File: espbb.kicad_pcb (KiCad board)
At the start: 2 copper layers, 20 x 20 mm, 10 parts, among them P1 CONN_8, P2 CONN_8, SW1 SWITCH_INV, U1 ESP-12/07v2/08v2, U2 LM6206

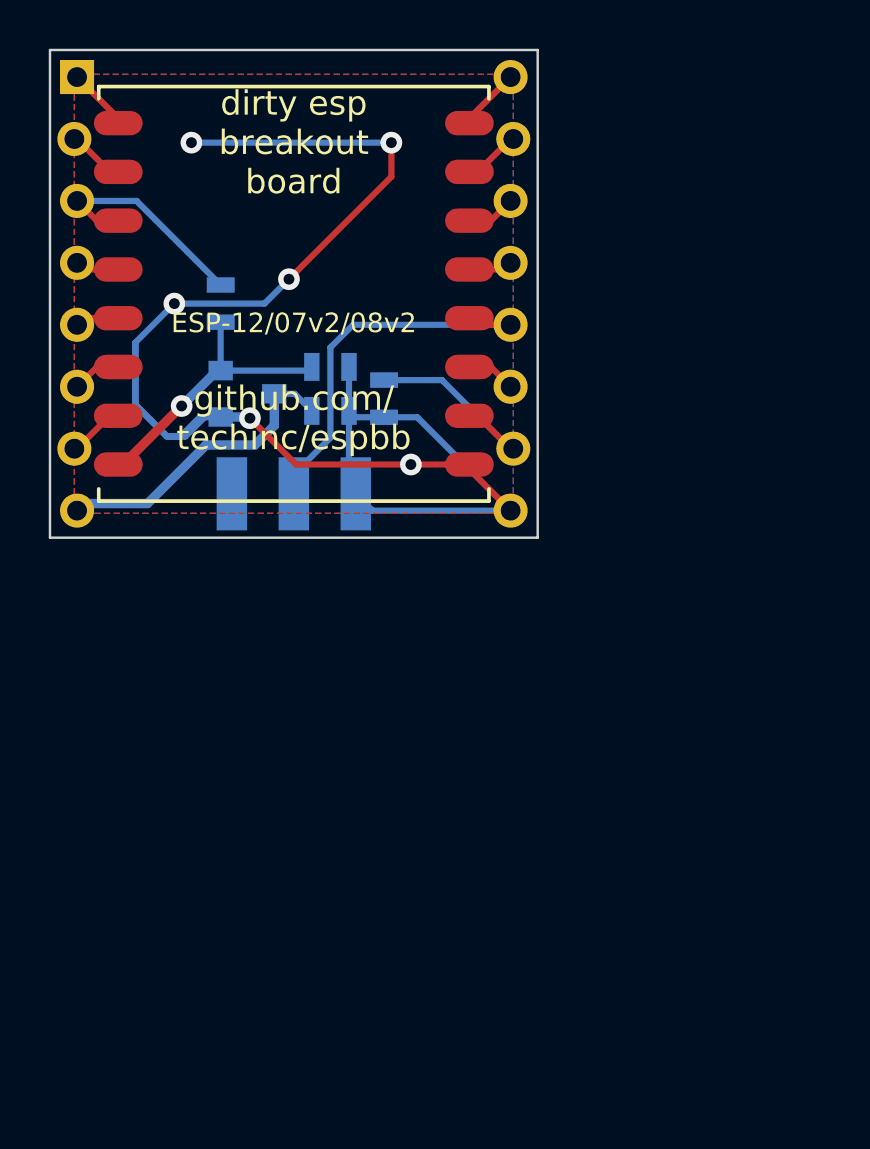
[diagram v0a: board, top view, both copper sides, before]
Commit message: esp-12e version
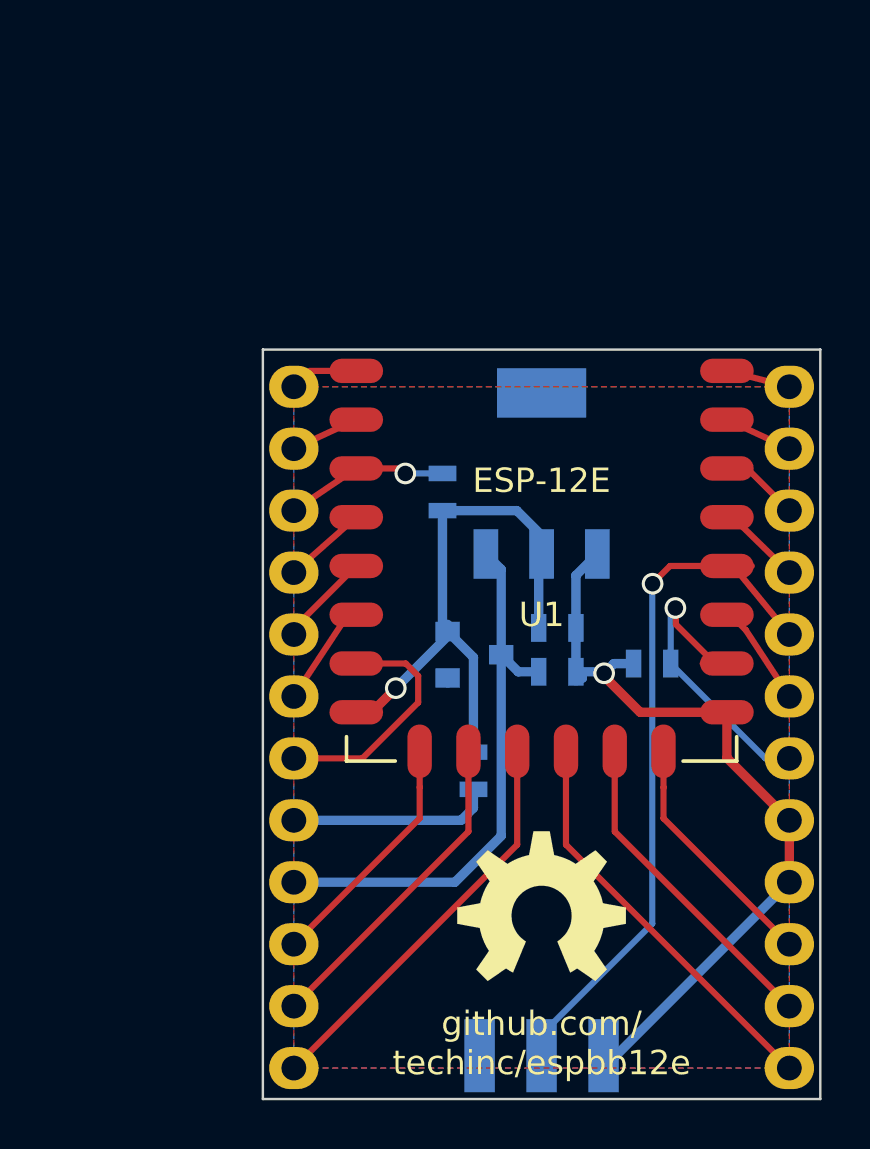
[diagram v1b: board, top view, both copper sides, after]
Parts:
- added R3: 0Ohm, r0603:SM0603, B.Cu at (7.37, 19.6)
- added U3: AMS1117-3.3, sot223:SOT223, B.Cu at (10.2, 7.37)
- ?: moved to F.Cu
- P1, P2: value CONN_8 -> CONN_01X12; footprint SIL-8 -> Pin_Headers:Pin_Header_Straight_1x12
- U1: value ESP-12/07v2/08v2 -> ESP-12E; footprint ESP-08v2 -> esp8266:ESP-12E
- moved P2 33.7 mm to (20.3, 31.8), turned to 180 degrees
- moved ? 31.2 mm to (10.2, 25.7), turned to 180 degrees
- moved SW1 25.2 mm to (10.2, 31.2)
- moved R2 15.5 mm to (14.7, 15.2), turned to 180 degrees
- moved U1 14.4 mm to (10.2, 10.2)
- moved C1 14.2 mm to (10.8, 13.7)
- moved C2 14.2 mm to (10.8, 15.5)
- moved U2 14.2 mm to (7.41, 14.8)
- moved R1 11.9 mm to (6.10, 8.13)
- moved P1 9.67 mm to (0.00, 3.81), turned to 0 degrees
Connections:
- P1 pad 8: VCC -> Net-(P1-Pad8)
- P2 pad 1: GND -> Net-(P2-Pad1)
- P2 pad 2: N-000009 -> Net-(P2-Pad2)
- P2 pad 3: N-000008 -> Net-(P2-Pad3)
- P2 pad 4: N-000007 -> GND
- P2 pad 5: N-000006 -> GND
- P2 pad 6: N-000005 -> Net-(P2-Pad6)
- P2 pad 7: N-000004 -> Net-(P2-Pad7)
- P2 pad 8: N-000001 -> Net-(P2-Pad8)
- R2 pad 1: N-000009 -> Net-(P2-Pad6)
- SW1 pad 1: (no net) -> Net-(SW1-Pad1)
- SW1 pad 2: N-000007 -> Net-(P2-Pad8)
- U1 pad 10: N-000009 -> Net-(P1-Pad11)
- U1 pad 11: N-000008 -> Net-(P1-Pad12)
- U1 pad 12: N-000007 -> Net-(P2-Pad1)
- U1 pad 13: N-000006 -> Net-(P2-Pad2)
- U1 pad 14: N-000005 -> Net-(P2-Pad3)
- U1 pad 15: N-000004 -> GND
- U1 pad 16: N-000001 -> Net-(P2-Pad6)
- U1 pad 9: GND -> Net-(P1-Pad10)
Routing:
- net GND: track 70.8 -> 34.2 mm, vias 6 -> 1
- net Net-(P2-Pad8): track 0.00 -> 30.5 mm, vias 0 -> 1
- net Net-(P2-Pad1): track 0.00 -> 16.8 mm
- net Net-(P1-Pad12): track 0.00 -> 16.8 mm
- net N-000007: track 16.2 -> 0.00 mm
- net 3V3: track 11.6 -> 26.9 mm
- net Net-(P2-Pad2): track 0.00 -> 13.4 mm
- net Net-(P1-Pad11): track 0.00 -> 13.4 mm
- net Net-(P2-Pad6): track 0.00 -> 13.3 mm, vias 0 -> 1
- net VCC: track 12.7 -> 22.9 mm
- net Net-(P2-Pad3): track 0.00 -> 9.65 mm
- net Net-(P1-Pad10): track 0.00 -> 9.65 mm
- net N-000009: track 8.60 -> 0.00 mm
- net Net-(P1-Pad8): track 0.00 -> 8.34 mm
- net Net-(P1-Pad7): track 2.25 -> 9.89 mm
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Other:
- board size 20 x 20 mm -> 22.9 x 30.7 mm
- board text added: "3V3 OUT"
- board text added: "CS0"
- board text added: "GPIO10"
- board text added: "GPIO9"
- board text added: "MISO"
- board text added: "MOSI"
- board text added: "SCLK"
- board text added: "github.com/ techinc/espbb12e"
- board text removed: "github.com/ techinc/espbb"
